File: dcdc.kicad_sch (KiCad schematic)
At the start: 48 parts, among them J10 Conn_01x01, J11 Conn_01x01, J12 Conn_01x01, J8 Conn_01x01, J9 Conn_01x01, T1 Transformer_SP_1S, U1 L78L33_SOT89, U2 TMP117, U3 LT3439, U6 LT3045xMSE

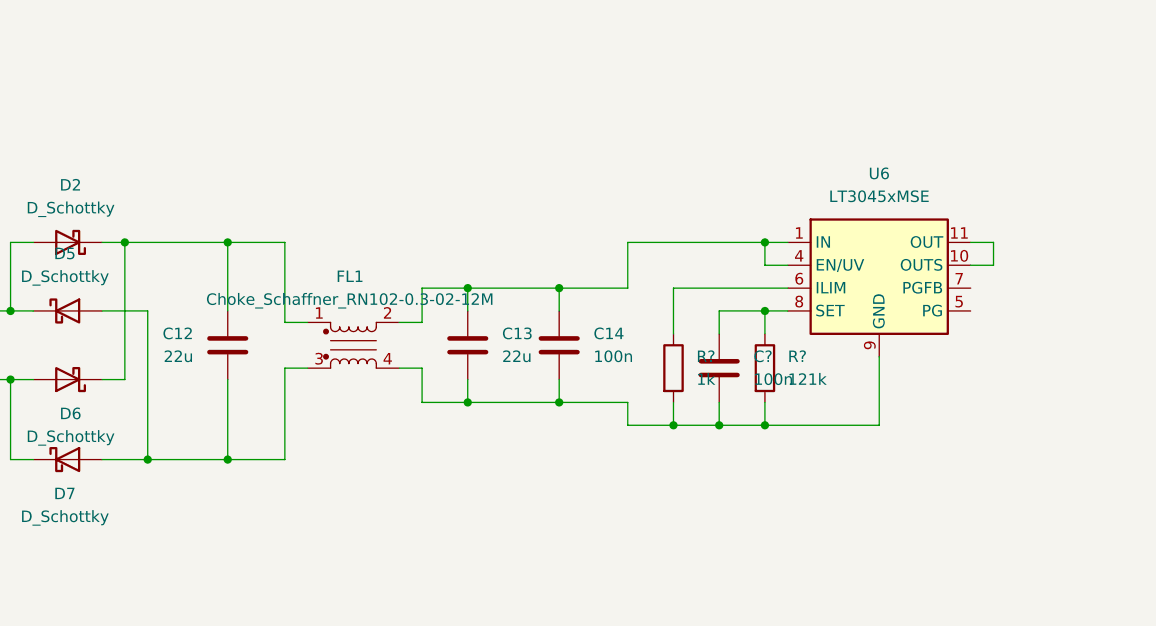
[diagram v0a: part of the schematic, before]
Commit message: asdf
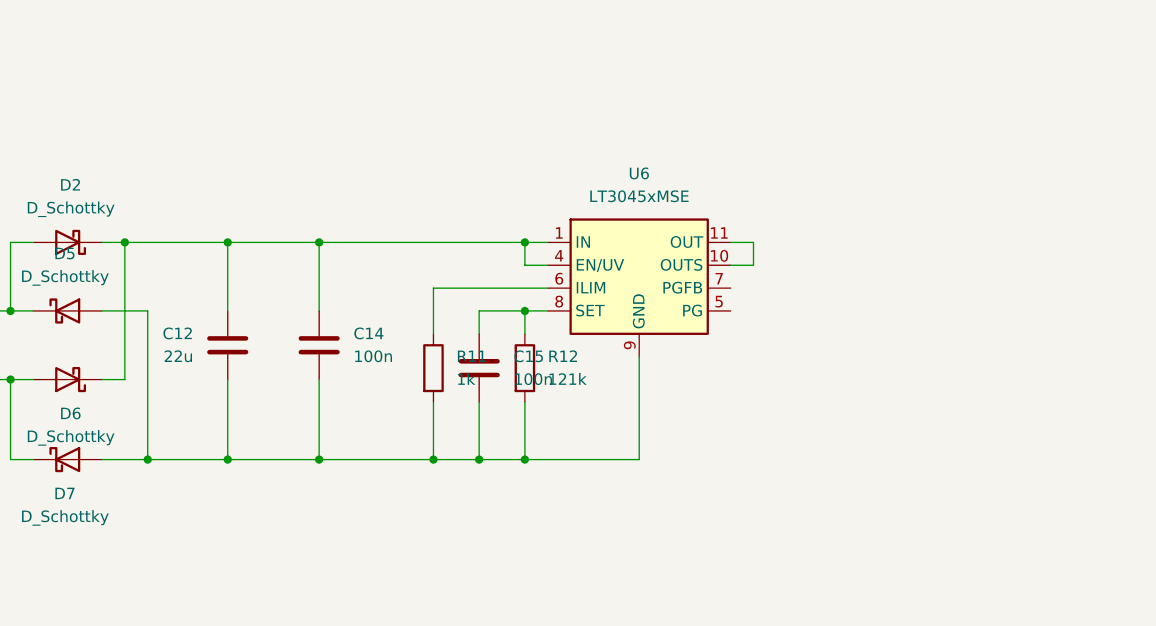
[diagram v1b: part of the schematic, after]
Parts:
- removed C13: 22u, Capacitor_SMD:C_1206_3216Metric, symbol Device:C
- removed FL1: Choke_Schaffner_RN102-0.3-02-12M, Inductor_THT:Choke_Schaffner_RN102-04-14.0x14.0mm, symbol Filter:Choke_Schaffner_RN102-0.3-02-12M
- gave numbers to parts that had none: 3
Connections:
- net at C12.1, D2.1 (K), D6.1 (K): now also C14.1, U6.1 (IN), U6.2 (IN), U6.3 (IN), U6.4 (EN/UV)
- net at C12.2, D5.2 (A), D7.2 (A): now also C14.2, C15.2, R11.2, R12.2, U6.13 (GND), U6.9 (GND)
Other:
- moved on the sheet: C14, C15, R11, R12, U6
